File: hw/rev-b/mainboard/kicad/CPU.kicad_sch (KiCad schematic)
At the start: 12 parts, among them SW1 RESET, SW2 NMI, U1 W65C02S, U2 IS62WV1288BLL-55QLI

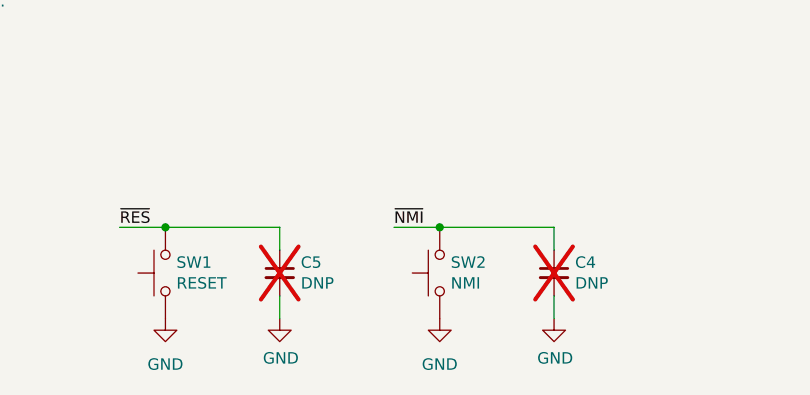
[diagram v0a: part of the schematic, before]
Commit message: chore(hw): tidy manufacturing files
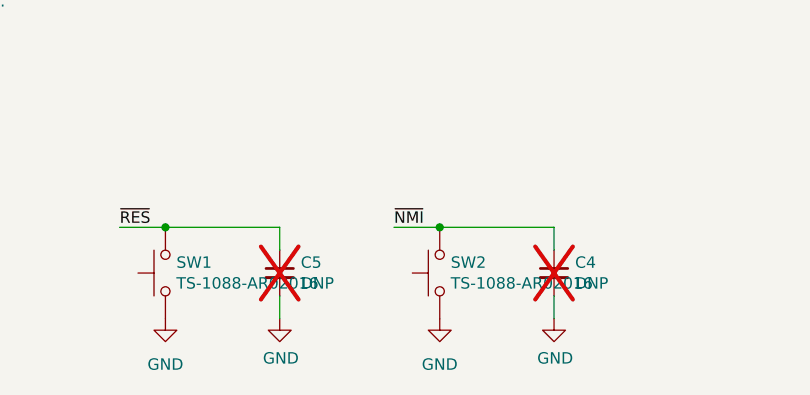
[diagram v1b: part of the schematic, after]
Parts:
- SW1: value RESET -> TS-1088-AR02016; MOUSER 611-PTS636SK43LFS -> (none)
- SW2: value NMI -> TS-1088-AR02016; MOUSER 611-PTS636SK43LFS -> (none)
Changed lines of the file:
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@@
 			)
 		)
-		(property "Value" "RESET"
+		(property "Value" "TS-1088-AR02016"
 			(at 96.4692 185.293 90)
 			(effects
@@
 			)
 		)
-		(property "MOUSER" "611-PTS636SK43LFS"
+		(property "MOUSER" ""
 			(at 95.25 184.15 0)
 			(effects
@@
 			)
 		)
-		(property "Value" "NMI"
+		(property "Value" "TS-1088-AR02016"
 			(at 126.9492 185.293 90)
 			(effects
@@
 			)
 		)
-		(property "MOUSER" "611-PTS636SK43LFS"
-			(at 125.73 184.15 0)
-			(effects
+		(property "MOUSER" ""
+			(at 125.73 184.15 0)
+			(effects

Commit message: chore(hw): create production files
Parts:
- C100, C104: LCSC C307331 -> (none); LCSC Part # (none) -> C307331
- R1, R2, R3, R4: LCSC C25900 -> (none); LCSC Part # (none) -> C25900
- SW1, SW2: LCSC C720477 -> (none); LCSC Part # (none) -> C720477
- U2: FT Rotation Offset (none) -> 90; LCSC C1351025 -> (none); LCSC Part # (none) -> C1351025
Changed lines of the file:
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@@
+			)
+		)
+		(property "FT Position Offset" ""
+			(at 92.71 106.68 0)
+			(effects
+				(font
+					(size 1.27 1.27)
+				)
+				(hide yes)
+			)
+		)
+		(property "FT Rotation Offset" ""
+			(at 92.71 106.68 0)
+			(effects
+				(font
+					(size 1.27 1.27)
+				)
+				(hide yes)
 			)
 		)
@@
 			)
 		)
-		(property "LCSC" "C1351025"
+		(property "LCSC Part #" "C1351025"
+			(at 187.96 97.79 0)
+			(effects
+				(font
+					(size 1.27 1.27)
+				)
+				(hide yes)
+			)
+		)
+		(property "FT Position Offset" ""
+			(at 187.96 97.79 0)
+			(effects
+				(font
+					(size 1.27 1.27)
+				)
+				(hide yes)
+			)
+		)
+		(property "FT Rotation Offset" "90"
 			(at 187.96 97.79 0)
 			(effects
@@
 			)
 		)
-		(property "LCSC" "C25900"
+		(property "LCSC Part #" "C25900"
+			(at 66.04 90.17 0)
+			(effects
+				(font
+					(size 1.27 1.27)
+				)
+				(hide yes)
+			)
+		)
+		(property "FT Position Offset" ""
+			(at 66.04 90.17 0)
+			(effects
+				(font
+					(size 1.27 1.27)
+				)
+				(hide yes)
+			)
+		)
+		(property "FT Rotation Offset" ""
 			(at 66.04 90.17 0)
 			(effects
@@
 			)
 		)
-		(property "LCSC" "C25900"
+		(property "LCSC Part #" "C25900"
+			(at 60.96 110.49 0)
+			(effects
+				(font
+					(size 1.27 1.27)
+				)
+				(hide yes)
+			)
+		)
+		(property "FT Position Offset" ""
+			(at 60.96 110.49 0)
+			(effects
+				(font
+					(size 1.27 1.27)
+				)
+				(hide yes)
+			)
+		)
+		(property "FT Rotation Offset" ""
 			(at 60.96 110.49 0)
 			(effects
@@
 			)
 		)
-		(property "LCSC" "C25900"
+		(property "LCSC Part #" "C25900"
+			(at 71.12 90.17 0)
+			(effects
+				(font
+					(size 1.27 1.27)
+				)
+				(hide yes)
+			)
+		)
+		(property "FT Position Offset" ""
+			(at 71.12 90.17 0)
+			(effects
+				(font
+					(size 1.27 1.27)
+				)
+				(hide yes)
+			)
+		)
+		(property "FT Rotation Offset" ""
 			(at 71.12 90.17 0)
 			(effects
@@
 			)
 		)
-		(property "LCSC" "C307331"
+		(property "LCSC Part #" "C307331"
+			(at 35.56 184.15 0)
+			(effects
+				(font
+					(size 1.27 1.27)
+				)
+				(hide yes)
+			)
+		)
+		(property "FT Position Offset" ""
+			(at 35.56 184.15 0)
+			(effects
+				(font
+					(size 1.27 1.27)
+				)
+				(hide yes)
+			)
+		)
+		(property "FT Rotation Offset" ""
 			(at 35.56 184.15 0)
 			(effects
@@
 			)
 		)
-		(property "LCSC" "C307331"
+		(property "LCSC Part #" "C307331"
+			(at 48.26 184.15 0)
+			(effects
+				(font
+					(size 1.27 1.27)
+				)
+				(hide yes)
+			)
+		)
+		(property "FT Position Offset" ""
+			(at 48.26 184.15 0)
+			(effects
+				(font
+					(size 1.27 1.27)
+				)
+				(hide yes)
+			)
+		)
+		(property "FT Rotation Offset" ""
 			(at 48.26 184.15 0)
 			(effects
@@
 			)
 		)
-		(property "LCSC" "C25900"
+		(property "LCSC Part #" "C25900"
+			(at 76.2 71.12 0)
+			(effects
+				(font
+					(size 1.27 1.27)
+				)
+				(hide yes)
+			)
+		)
+		(property "FT Position Offset" ""
+			(at 76.2 71.12 0)
+			(effects
+				(font
+					(size 1.27 1.27)
+				)
+				(hide yes)
+			)
+		)
+		(property "FT Rotation Offset" ""
 			(at 76.2 71.12 0)
 			(effects
@@
 			)
 		)
-		(property "LCSC" ""
+		(property "FT Position Offset" ""
+			(at 107.95 184.15 0)
+			(effects
+				(font
+					(size 1.27 1.27)
+				)
+				(hide yes)
+			)
+		)
+		(property "FT Rotation Offset" ""
 			(at 107.95 184.15 0)
 			(effects
@@
 			)
 		)
-		(property "LCSC" "C720477"
+		(property "LCSC Part #" "C720477"
+			(at 95.25 184.15 0)
+			(effects
+				(font
+					(size 1.27 1.27)
+				)
+				(hide yes)
+			)
+		)
+		(property "FT Position Offset" ""
+			(at 95.25 184.15 0)
+			(effects
+				(font
+					(size 1.27 1.27)
+				)
+				(hide yes)
+			)
+		)
+		(property "FT Rotation Offset" ""
 			(at 95.25 184.15 0)
 			(effects
@@
 			)
 		)
-		(property "LCSC" "C720477"
+		(property "LCSC Part #" "C720477"
+			(at 125.73 184.15 0)
+			(effects
+				(font
+					(size 1.27 1.27)
+				)
+				(hide yes)
+			)
+		)
+		(property "FT Position Offset" ""
+			(at 125.73 184.15 0)
+			(effects
+				(font
+					(size 1.27 1.27)
+				)
+				(hide yes)
+			)
+		)
+		(property "FT Rotation Offset" ""
 			(at 125.73 184.15 0)
 			(effects
@@
 			)
 		)
-		(property "LCSC" ""
+		(property "FT Position Offset" ""
 			(at 138.43 184.15 0)
 			(effects
+				(font
+					(size 1.27 1.27)
+				)
+				(hide yes)
+			)
+		)
+		(property "FT Rotation Offset" ""
+			(at 138.43 184.15 0)
+			(effects
